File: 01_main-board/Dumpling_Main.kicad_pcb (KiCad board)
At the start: 4 copper layers, 75 x 135.2 mm, 354 parts, among them J1 Conn_ARM_SWD_TagConnect_TC203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, J10 MICROMOD-2222-C, J11 USB_C_Receptacle_USB2.0_16P, J12 Conn_ARM_SWD_TagConnect_TC203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, J13 MICROMOD-2222-C, J14 USB_C_Receptacle_USB2.0_16P, J15 Conn_ARM_SWD_TagConnect_TC203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, J16 MICROMOD-2222-C, J17 USB_C_Receptacle_USB2.0_16P, J18 Conn_ARM_SWD_TagConnect_TC203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, J19 MICROMOD-2222-C, J2 Micro_SD_Card, J20 USB_C_Receptacle_USB2.0_16P, J21 Conn_ARM_SWD_TagConnect_TC203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, J22 MICROMOD-2222-C, J23 USB_C_Receptacle_USB2.0_16P, J3 USB_C_Receptacle_USB2.0_16P, J4 XT30PW-M, J5 SM04B-SRSS-TB, J6 Conn_ARM_SWD_TagConnect_TC203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, J7 MICROMOD-2222-C, J8 USB_C_Receptacle_USB2.0_16P, J9 Conn_ARM_SWD_TagConnect_TC203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, Q1 AO3401A, Q2 S8050, SW1 SW_DPST, SW10 SW_SPDT, SW11 SW_DPST, SW12 SW_SPDT, SW13 SW_DPST, SW14 SW_SPDT, SW2 SW_DPST, SW3 SW_DPST, SW4 SW_SPDT, SW5 SW_DPST, SW6 SW_SPDT, SW7 SW_DPST, SW8 SW_SPDT, SW9 SW_DPST, U1 STM32F405RGTx, U10 W25Q128JVS, U11 USBLC6-2SC6, U12 W25Q128JVS, U13 STM32F411CEUx, U14 USBLC6-2SC6, U15 W25Q128JVS, U16 STM32F411CEUx, U17 USBLC6-2SC6, U18 W25Q128JVS, U19 STM32F411CEUx, U2 USBLC6-2SC6, U20 USBLC6-2SC6, U22 STM32F411CEUx, U23 USBLC6-2SC6, U24 W25Q128JVS, U25 TPS562200, U26 TPS562200, U3 W25Q128JVS, U4 STM32F411CEUx, U5 STM32F411CEUx, U6 USBLC6-2SC6, U8 W25Q128JVS, U9 INA219AxDCN, Y1 32.768kHz, Y2 32.768kHz, Y3 32.768kHz, Y4 32.768kHz, Y5 32.768kHz, Y6 32.768kHz, Y7 32.768kHz

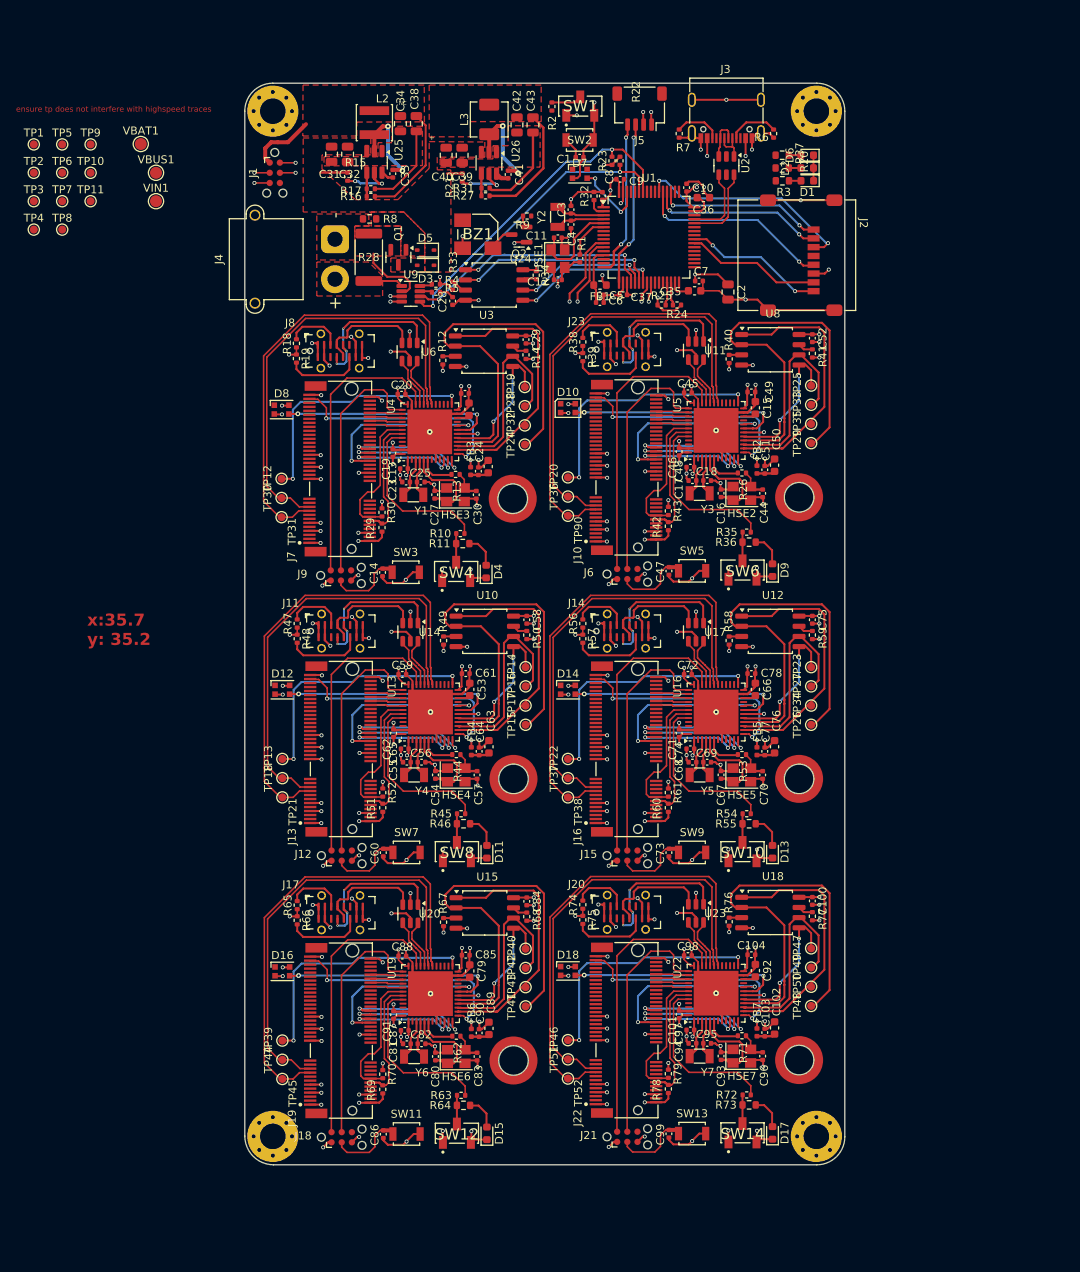
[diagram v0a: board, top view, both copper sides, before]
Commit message: wired
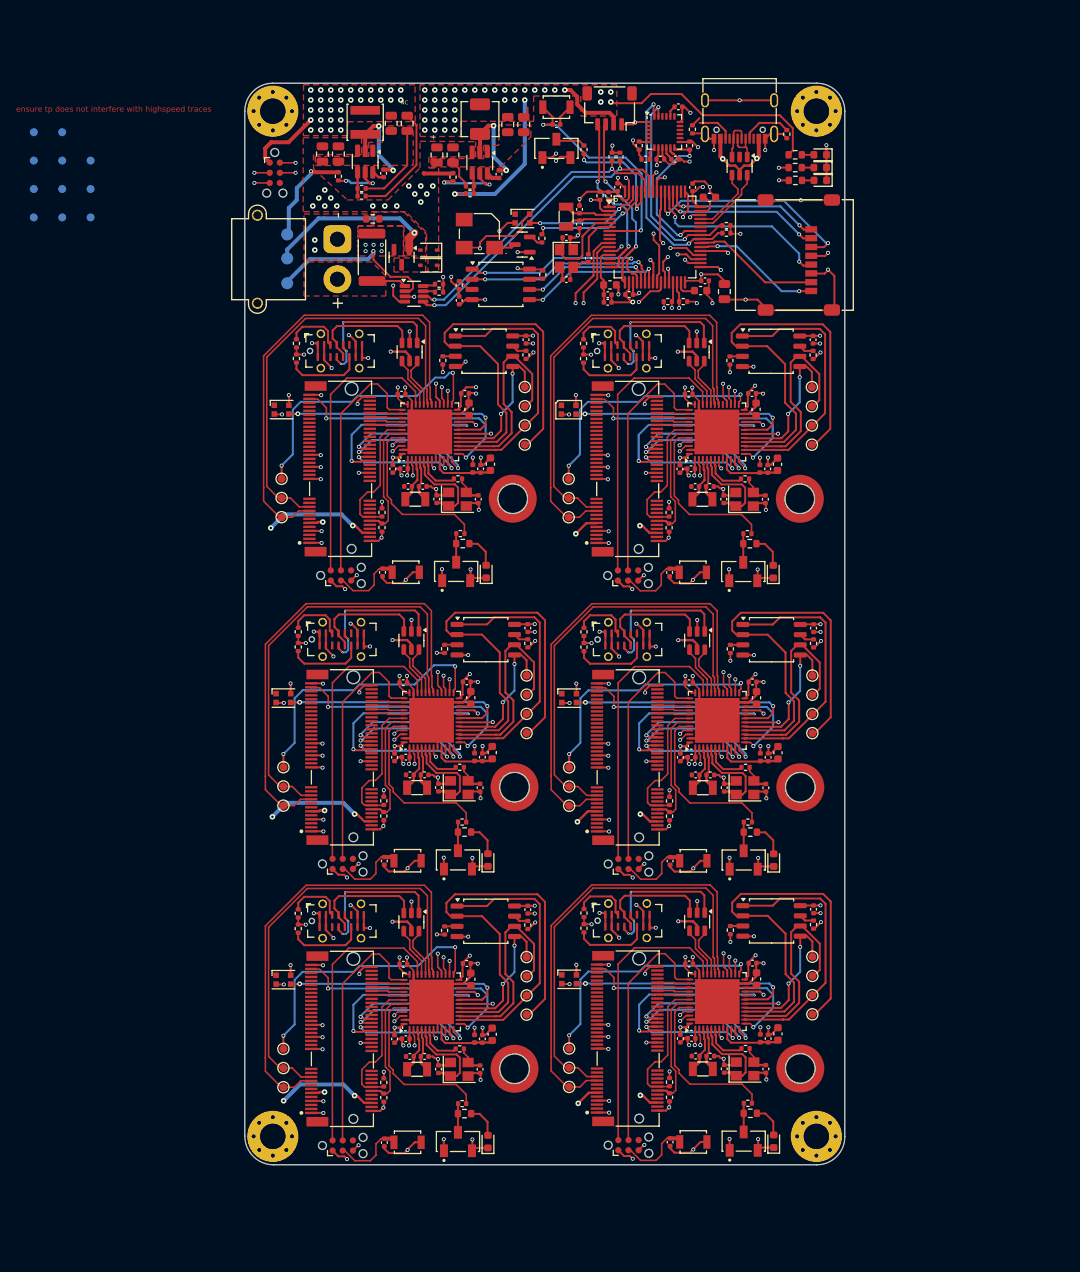
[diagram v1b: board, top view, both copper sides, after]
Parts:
- added C105: 10n, Capacitor_SMD:C_0402_1005Metric, F.Cu at (145.4, 53.9)
- added C106: 0.22u, Capacitor_SMD:C_0402_1005Metric, F.Cu at (147.3, 53.9)
- added C107: 0.22u, Capacitor_SMD:C_0402_1005Metric, F.Cu at (147.7, 47.4)
- added R80: 4.7k, Resistor_SMD:R_0402_1005Metric, F.Cu at (153.7, 63.1)
- added R81: 4.7k, Resistor_SMD:R_0402_1005Metric, F.Cu at (153.7, 62.2)
- added R82: 5.1k, Resistor_SMD:R_0402_1005Metric, F.Cu at (142.8, 52.2)
- added R83: 5.1k, Resistor_SMD:R_0402_1005Metric, F.Cu at (143.6, 53.9)
- added R84: 10k, Resistor_SMD:R_0402_1005Metric, F.Cu at (149.1, 52.2)
- added U7: MPU-6050, Sensor_Motion:InvenSense_QFN-24_4x4mm_P0.5mm, F.Cu at (145.9, 50.5)
- TP1, TP10, TP11, TP2, TP3, TP4, TP5, TP6, TP7, TP8, TP9, VBAT1, VBUS1, VIN1: moved to B.Cu
- moved VBAT1 25.3 mm to (98.8, 69.4)
- moved C100 23.8 mm to (147.9, 163.8)
- moved C84 22.9 mm to (113.6, 163.8), turned to 180 degrees
- moved C58 22.9 mm to (113.6, 128.6), turned to 180 degrees
- moved C62 21.5 mm to (128.9, 112.5), turned to -90 degrees
- moved C91 21.5 mm to (128.9, 147.7), turned to -90 degrees
- moved C97 21.3 mm to (164.6, 147.7), turned to -90 degrees
- moved VBUS1 19.6 mm to (98.8, 66.3)
- moved VIN1 16.9 mm to (98.8, 63.3)
- moved C78 13.7 mm to (147.9, 128.7), turned to -90 degrees
- moved C49 13.1 mm to (147.9, 92.6), turned to -90 degrees
- moved TP4 12.2 mm to (67.1, 50.5)
- moved TP8 12.2 mm to (70.7, 50.5)
- moved C46 12.0 mm to (156.9, 83.2), turned to 0 degrees
- moved C71 11.4 mm to (157.0, 119.2), turned to 0 degrees
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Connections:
- J2 pad 8: SDIO_D1 -> SDIO_D7
- U1 pad 38: unconnected-(U1-PC7-Pad38) -> SDIO_D7
- U1 pad 40: SDIO_D1 -> I2C3_SDA
- U1 pad 41: unconnected-(U1-PA8-Pad41) -> I2C3_SCL
- U1 pad 42: unconnected-(U1-PA9-Pad42) -> IMU_INT
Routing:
- net SPI2_MOSI: track 0.00 -> 243.7 mm, vias 0 -> 7
- net SPI2_SCK: track 0.00 -> 238.8 mm, vias 0 -> 7
- net SPI2_MISO: track 0.00 -> 238.5 mm, vias 0 -> 7
- net I2C2_SCL: track 3.06 -> 230.1 mm, vias 0 -> 7
- net Trigger: track 17.7 -> 241.9 mm, vias 6 -> 7
- net I2C2_SDA: track 2.90 -> 214.8 mm, vias 0 -> 7
- net co5_NRST: track 9.70 -> 168.9 mm, vias 0 -> 2
- net +5V: track 25.4 -> 173.2 mm, vias 7 -> 48
- net SPI2_NSS5: track 34.5 -> 178.2 mm
- net co6_NRST: track 9.70 -> 140.6 mm, vias 0 -> 2
- net SPI2_NSS6: track 34.3 -> 148.9 mm
- net co3_NRST: track 9.70 -> 117.4 mm, vias 0 -> 2
- net VBUS: track 57.7 -> 162.3 mm, vias 20 -> 21
- net co4_NRST: track 9.70 -> 98.8 mm, vias 0 -> 2
- net SPI2_NSS3: track 41.5 -> 122.4 mm
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- added copper zone on In2.Cu, net +3V3
- added copper zone on In2.Cu, net +5V
- added copper zone on In2.Cu, net VBUS
- added copper zone on In2.Cu, net VIN
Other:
- copper layers 4 -> 6
- board text added: "change switch, import 3d model, tp, Cu fill vias -> run drc -> label components"
- board text added: "no copper directly below component"
- board text removed: "RxTx"
- board text removed: "i2c1:INA"
- board text removed: "spi1:flsh"
- board text removed: "x:35.7 y: 35.2"

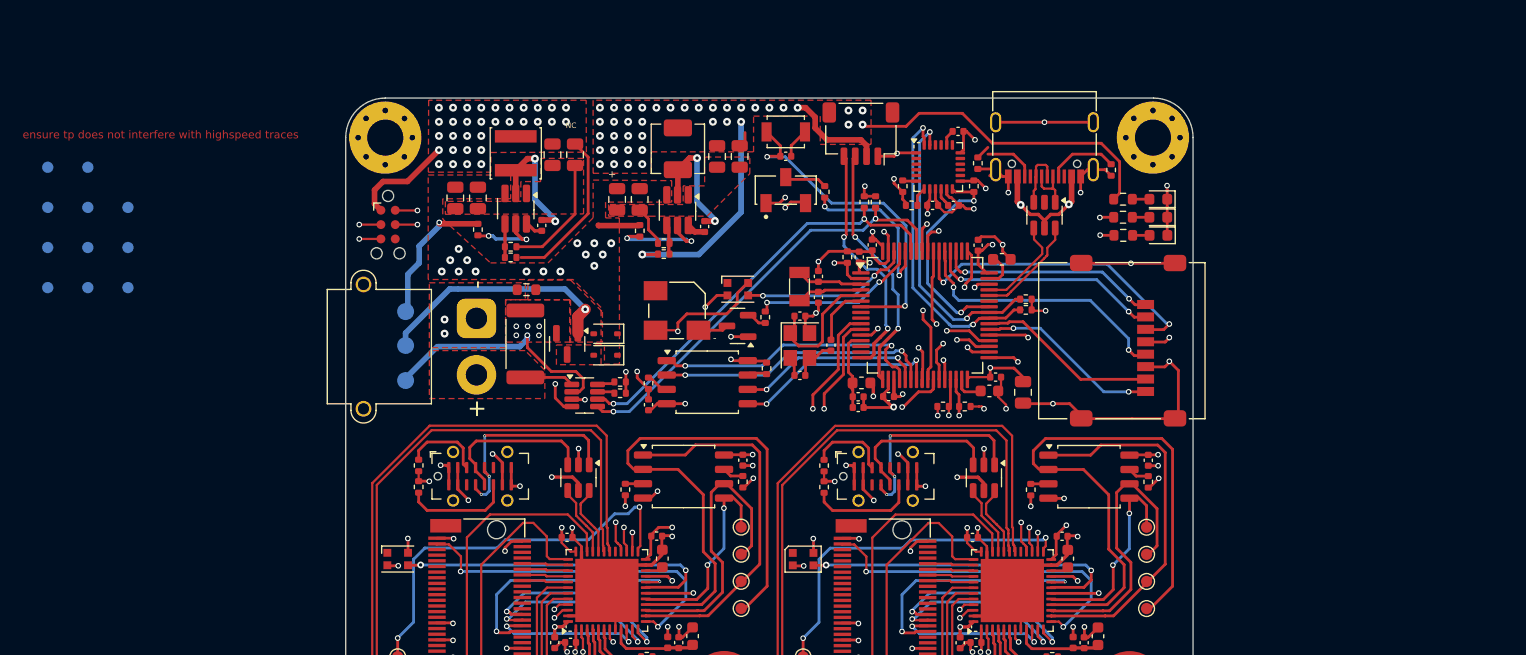
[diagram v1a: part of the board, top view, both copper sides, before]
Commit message: wiring fin, pre-drc
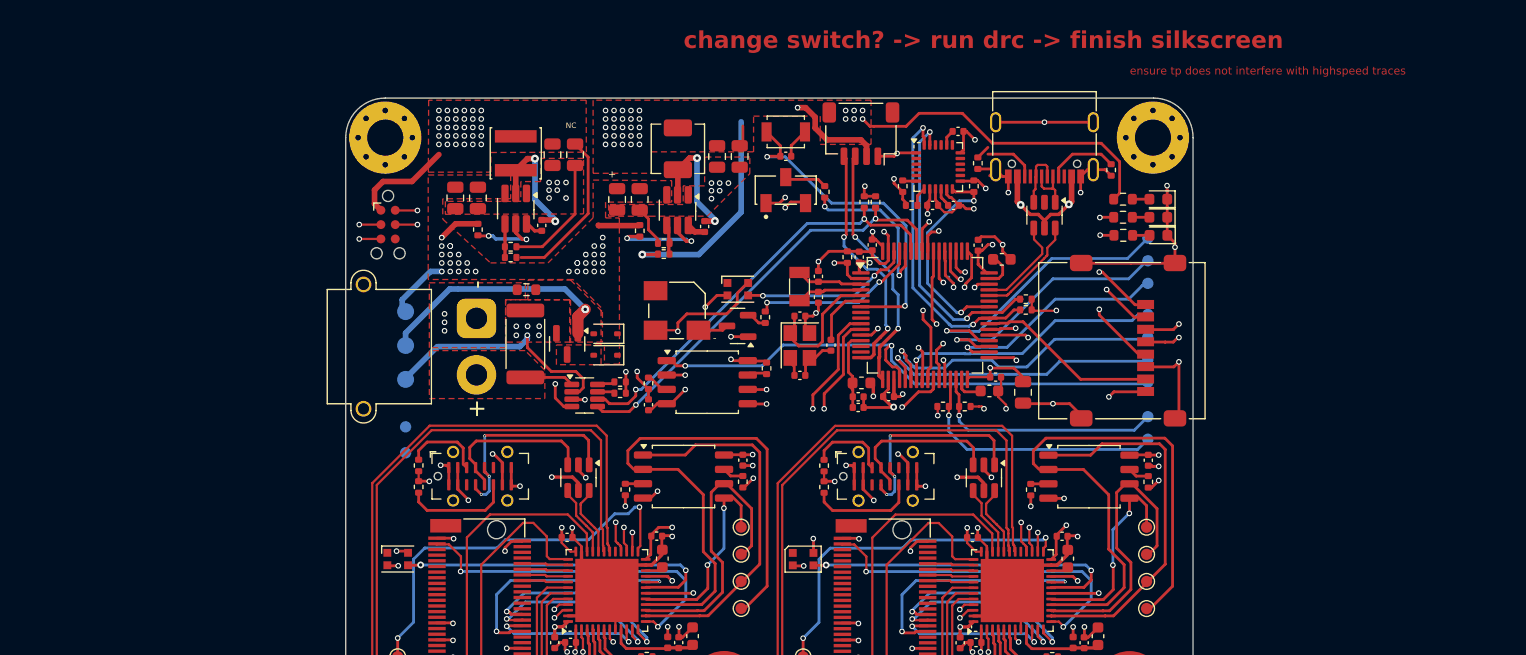
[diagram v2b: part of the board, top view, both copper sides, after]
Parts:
- moved TP4 100.3 mm to (164.5, 74.6)
- moved TP3 99.1 mm to (164.5, 72.6)
- moved TP8 95.7 mm to (164.5, 69.5), turned to 180 degrees
- moved TP7 94.8 mm to (164.5, 67.5), turned to 180 degrees
- moved TP6 94.2 mm to (164.5, 65.5), turned to 180 degrees
- moved TP5 93.9 mm to (164.5, 63.5), turned to 180 degrees
- moved TP11 90.5 mm to (164.5, 60.8), turned to 180 degrees
- moved TP9 90.4 mm to (164.5, 56.8), turned to 180 degrees
- moved TP10 90.3 mm to (164.5, 58.8), turned to 180 degrees
- moved TP2 36.5 mm to (98.8, 75.8), turned to 180 degrees
- moved TP1 34.0 mm to (98.8, 73.5), turned to 180 degrees
- moved VBAT1 0.10 mm to (98.8, 69.3)
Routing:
- net SPI1_NSS: track 25.0 -> 50.0 mm
- net SPI1_MISO: track 24.5 -> 48.8 mm
- net SPI1_SCK: track 16.9 -> 40.2 mm
- net SPI1_MOSI: track 18.3 -> 40.5 mm
- net SPI2_MOSI: track 243.7 -> 264.9 mm
- net I2C2_SCL: track 230.1 -> 250.1 mm
- net SPI2_MISO: track 238.5 -> 258.3 mm
- net SPI2_SCK: track 238.8 -> 257.1 mm
- net I2C2_SDA: track 214.8 -> 232.9 mm
- net GND: track 469.8 -> 465.1 mm, vias 164 -> 178
- net VIN: track 89.5 -> 86.4 mm, vias 22 -> 38
- net SDIO_CMD: track 27.8 -> 29.5 mm
- net co6_NRST: track 140.6 -> 138.9 mm
- net +3V3: track 246.0 -> 247.3 mm, vias 136 -> 134
- net +5V: track 173.2 -> 174.2 mm, vias 48 -> 42
- added copper zone on In1.Cu, net GND
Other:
- board text added: "change switch? -> run drc -> finish silkscreen"
- board text removed: "change switch, import 3d model, tp, Cu fill vias -> run drc -> label components"
